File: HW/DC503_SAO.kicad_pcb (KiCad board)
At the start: 2 copper layers, 54.9 x 39.2 mm, 28 parts, among them J1 GS2, J2 GS2, U1 ATTINY85-20SU, X1 Badgelife_shitty_connector

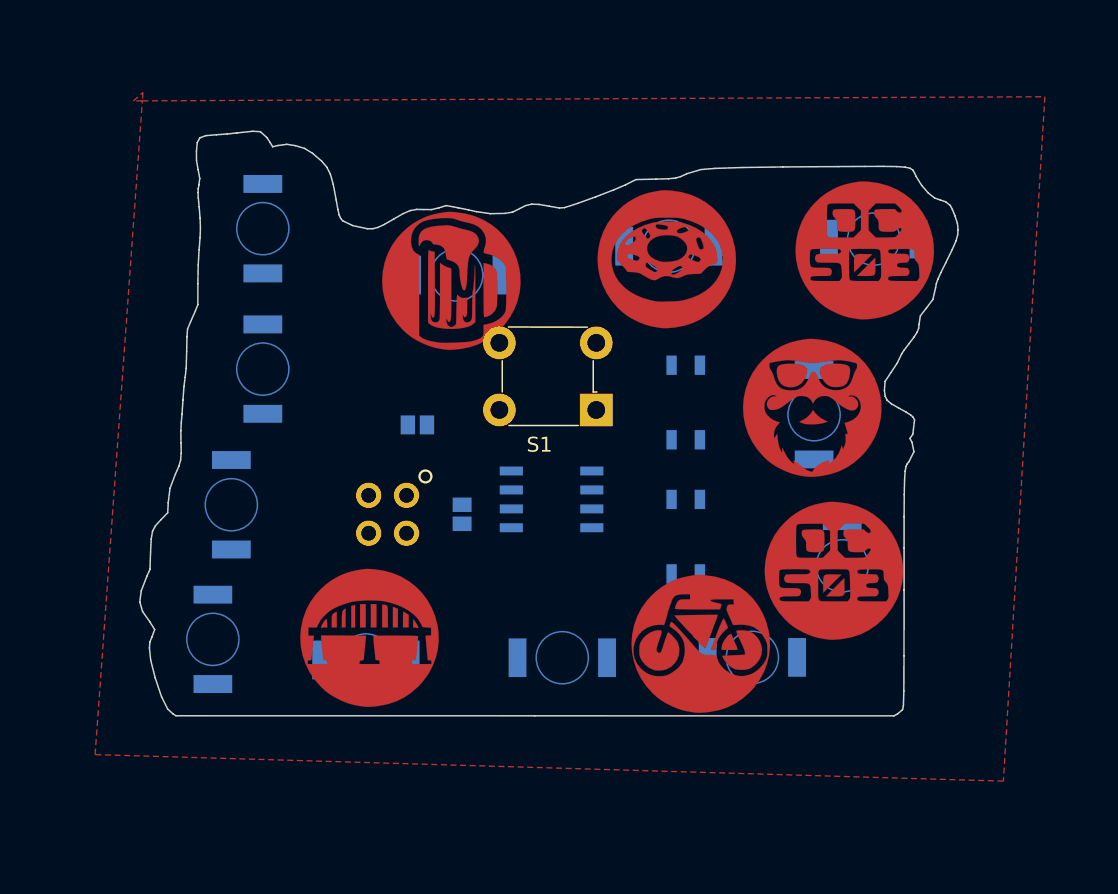
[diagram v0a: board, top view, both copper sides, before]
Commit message: finialized art
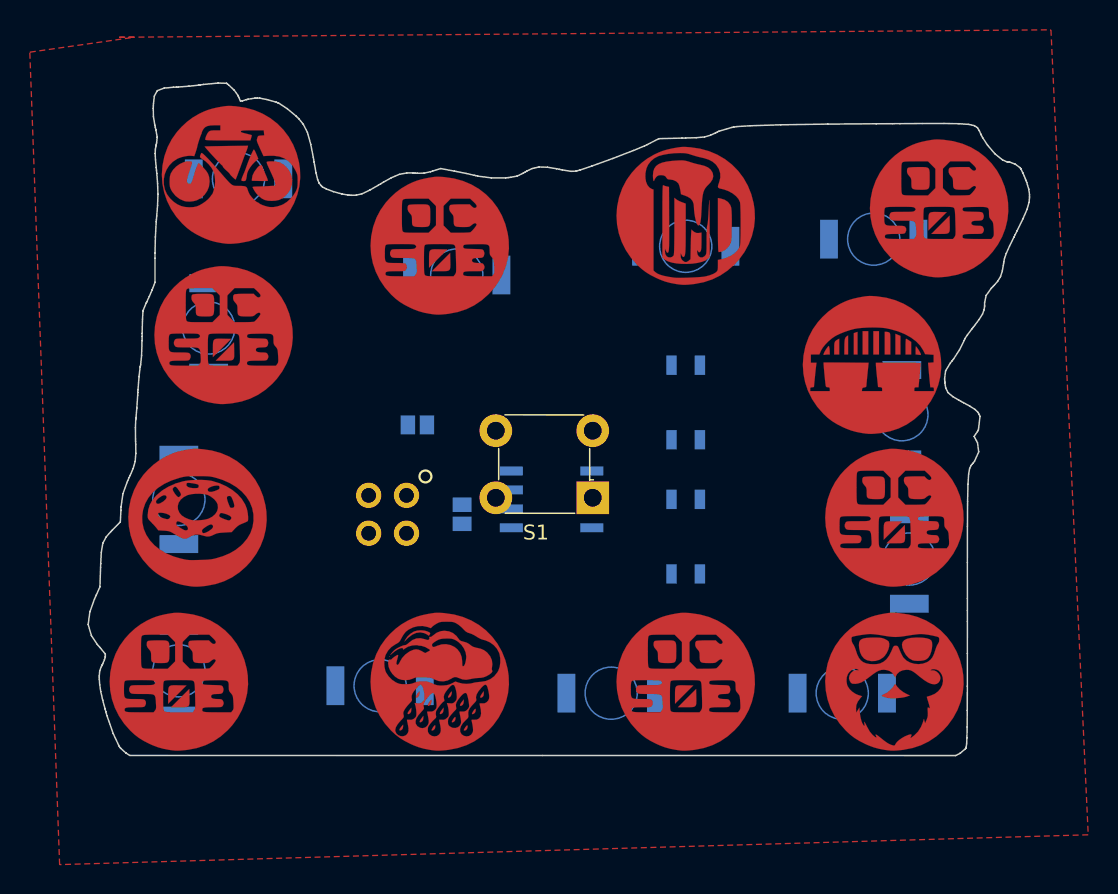
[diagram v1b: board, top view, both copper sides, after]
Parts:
- removed the G*** at (192.9, 96.8)
- added G***: LOGO, DC503_SAO:DC_503, F.Cu at (183.0, 104.2)
- added G***: LOGO, DC503_SAO:DC_503, F.Cu at (149.0, 104.2)
- added G***: LOGO, DC503_SAO:DC_503, F.Cu at (197.0, 93.2)
- added G***: LOGO, DC503_SAO:DC_503, F.Cu at (200.0, 72.5)
- added G***: LOGO, DC503_SAO:rain, F.Cu at (166.5, 104.2)
- added G***: LOGO, DC503_SAO:heart, F.Cu at (174.6, 124.4)
- added G***: LOGO, DC503_SAO:DC_503, F.Cu at (152.0, 81.0)
- X1: footprint DC503_SAO:Badgelife-Shitty-2x2 -> Badgelife-Shitty-2x2
- moved G*** 44.5 mm to (152.5, 70.2)
- moved G*** 38.4 mm to (195.5, 83.0)
- moved G*** 35.9 mm to (150.2, 93.2)
- moved G*** 28.5 mm to (166.5, 75.0)
- moved G*** 19.2 mm to (197.0, 104.2)
- moved G*** 16.3 mm to (183.0, 73.0)
- moved D7 6.49 mm to (193.5, 105.0)
- moved S1 5.89 mm to (176.8, 91.9)
- moved D5 5.89 mm to (197.5, 86.3)
- moved D12 4.56 mm to (151.0, 80.5)
- moved D6 4.52 mm to (198.0, 96.0)
- moved D8 4.05 mm to (178.0, 105.0)
- moved D1 3.72 mm to (153.0, 70.5), turned to 180 degrees
- moved D11 3.54 mm to (149.0, 92.0)
- moved D10 3.11 mm to (149.0, 103.5)
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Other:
- board size 54.9 x 39.2 mm -> 63.1 x 45.1 mm
